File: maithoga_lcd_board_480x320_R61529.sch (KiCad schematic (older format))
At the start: 0 parts

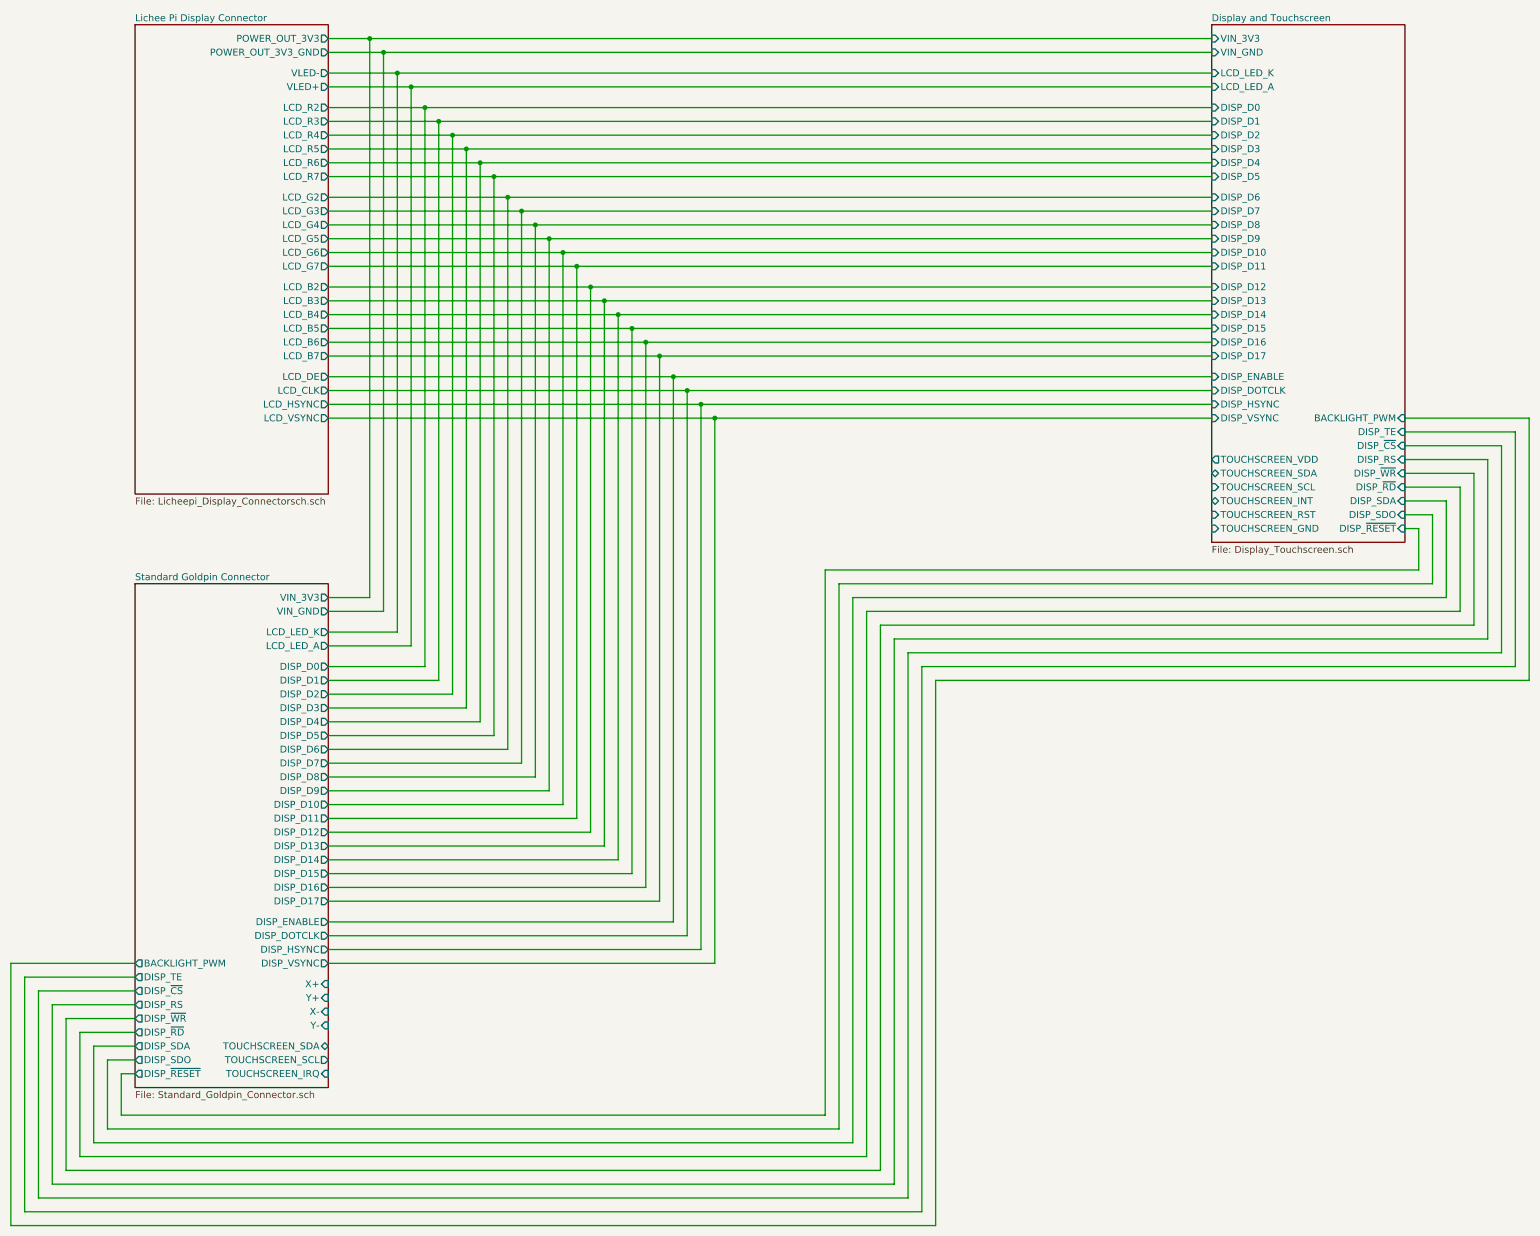
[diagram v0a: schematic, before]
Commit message: Generated gerbers
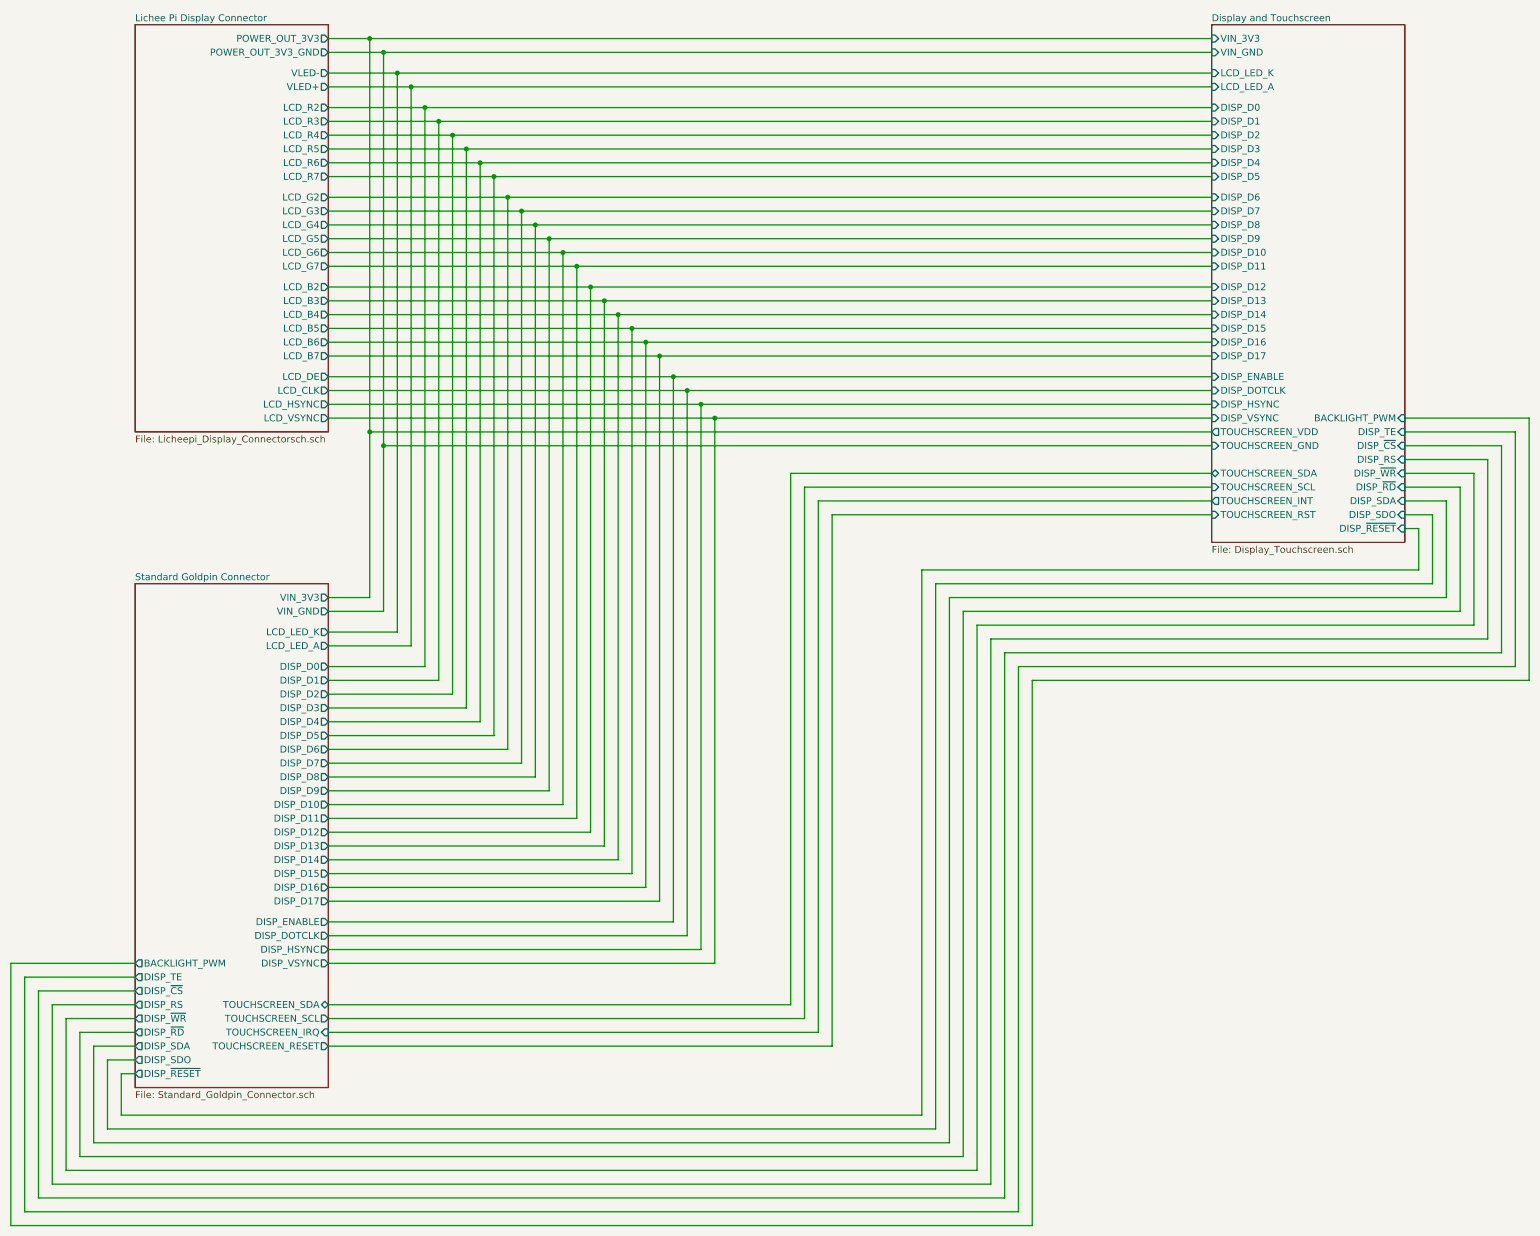
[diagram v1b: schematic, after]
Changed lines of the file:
@@
 F35 "LCD_LED_K" I L 11750 1800 50
 F36 "LCD_LED_A" I L 11750 1900 50
-F37 "TOUCHSCREEN_VDD" O L 11750 4600 50
+F37 "TOUCHSCREEN_VDD" O L 11750 4400 50
 F38 "TOUCHSCREEN_SDA" B L 11750 4700 50
 F39 "TOUCHSCREEN_SCL" I L 11750 4800 50
-F40 "TOUCHSCREEN_INT" B L 11750 4900 50
-F41 "TOUCHSCREEN_RST" I L 11750 5000 50
-F42 "TOUCHSCREEN_GND" I L 11750 5100 50
+F40 "TOUCHSCREEN_RST" I L 11750 5000 50
+F41 "TOUCHSCREEN_GND" I L 11750 4500 50
+F42 "TOUCHSCREEN_INT" O L 11750 4900 50
 $EndSheet
 $Sheet
@@
 F0 "Standard Goldpin Connector" 50
 F1 "Standard_Goldpin_Connector.sch" 50
-F2 "TOUCHSCREEN_IRQ" I R 5350 9050 50
-F3 "TOUCHSCREEN_SDA" B R 5350 8850 50
-F4 "TOUCHSCREEN_SCL" O R 5350 8950 50
-F5 "VIN_3V3" O R 5350 5600 50
-F6 "VIN_GND" O R 5350 5700 50
-F7 "BACKLIGHT_PWM" O L 3950 8250 50
-F8 "DISP_TE" O L 3950 8350 50
-F9 "DISP_~CS~" O L 3950 8450 50
-F10 "DISP_RS" O L 3950 8550 50
-F11 "DISP_~WR~" O L 3950 8650 50
-F12 "DISP_~RD~" O L 3950 8750 50
-F13 "DISP_SDA" O L 3950 8850 50
-F14 "DISP_SDO" O L 3950 8950 50
-F15 "DISP_D0" O R 5350 6100 50
-F16 "DISP_D1" O R 5350 6200 50
-F17 "DISP_D2" O R 5350 6300 50
-F18 "DISP_D3" O R 5350 6400 50
-F19 "DISP_D4" O R 5350 6500 50
-F20 "DISP_D5" O R 5350 6600 50
-F21 "DISP_D6" O R 5350 6700 50
-F22 "DISP_D7" O R 5350 6800 50
-F23 "DISP_D8" O R 5350 6900 50
-F24 "DISP_D9" O R 5350 7000 50
-F25 "DISP_D10" O R 5350 7100 50
-F26 "DISP_D11" O R 5350 7200 50
-F27 "DISP_D12" O R 5350 7300 50
-F28 "DISP_D13" O R 5350 7400 50
-F29 "DISP_D14" O R 5350 7500 50
-F30 "DISP_D15" O R 5350 7600 50
-F31 "DISP_D16" O R 5350 7700 50
-F32 "DISP_D17" O R 5350 7800 50
-F33 "DISP_ENABLE" O R 5350 7950 50
-F34 "DISP_DOTCLK" O R 5350 8050 50
-F35 "DISP_HSYNC" O R 5350 8150 50
-F36 "DISP_VSYNC" O R 5350 8250 50
-F37 "DISP_~RESET~" O L 3950 9050 50
-F38 "LCD_LED_K" O R 5350 5850 50
-F39 "LCD_LED_A" O R 5350 5950 50
-F40 "X-" I R 5350 8600 50
-F41 "X+" I R 5350 8400 50
-F42 "Y-" I R 5350 8700 50
-F43 "Y+" I R 5350 8500 50
+F2 "VIN_3V3" O R 5350 5600 50
+F3 "VIN_GND" O R 5350 5700 50
+F4 "BACKLIGHT_PWM" O L 3950 8250 50
+F5 "DISP_TE" O L 3950 8350 50
+F6 "DISP_~CS~" O L 3950 8450 50
+F7 "DISP_RS" O L 3950 8550 50
+F8 "DISP_~WR~" O L 3950 8650 50
+F9 "DISP_~RD~" O L 3950 8750 50
+F10 "DISP_SDA" O L 3950 8850 50
+F11 "DISP_SDO" O L 3950 8950 50
+F12 "DISP_D0" O R 5350 6100 50
+F13 "DISP_D1" O R 5350 6200 50
+F14 "DISP_D2" O R 5350 6300 50
+F15 "DISP_D3" O R 5350 6400 50
+F16 "DISP_D4" O R 5350 6500 50
+F17 "DISP_D5" O R 5350 6600 50
+F18 "DISP_D6" O R 5350 6700 50
+F19 "DISP_D7" O R 5350 6800 50
+F20 "DISP_D8" O R 5350 6900 50
+F21 "DISP_D9" O R 5350 7000 50
+F22 "DISP_D10" O R 5350 7100 50
+F23 "DISP_D11" O R 5350 7200 50
+F24 "DISP_D12" O R 5350 7300 50
+F25 "DISP_D13" O R 5350 7400 50
+F26 "DISP_D14" O R 5350 7500 50
+F27 "DISP_D15" O R 5350 7600 50
+F28 "DISP_D16" O R 5350 7700 50
+F29 "DISP_D17" O R 5350 7800 50
+F30 "DISP_ENABLE" O R 5350 7950 50
+F31 "DISP_DOTCLK" O R 5350 8050 50
+F32 "DISP_HSYNC" O R 5350 8150 50
+F33 "DISP_VSYNC" O R 5350 8250 50
+F34 "DISP_~RESET~" O L 3950 9050 50
+F35 "LCD_LED_K" O R 5350 5850 50
+F36 "LCD_LED_A" O R 5350 5950 50
+F37 "TOUCHSCREEN_IRQ" I R 5350 8750 50
+F38 "TOUCHSCREEN_SDA" B R 5350 8550 50
+F39 "TOUCHSCREEN_SCL" O R 5350 8650 50
+F40 "TOUCHSCREEN_RESET" O R 5350 8850 50
 $EndSheet
 $Sheet
-S 3950 1450 1400 3400
+S 3950 1450 1400 2950
 U 5F06906E
 F0 "Lichee Pi Display Connector" 50
@@
 Wire Wire Line
 	5350 5600 5650 5600
-Wire Wire Line
-	5650 5600 5650 1550
 Connection ~ 5650 1550
 Wire Wire Line
 	5650 1550 11750 1550
 Wire Wire Line
-	5750 1650 5750 5700
+	5750 1650 5750 4500
 Wire Wire Line
 	5750 5700 5350 5700
@@
 	13250 5100 13250 5400
 Wire Wire Line
-	8950 5400 8950 9350
-Wire Wire Line
-	8950 9350 3850 9350
+	9650 5400 9650 9350
+Wire Wire Line
+	9650 9350 3850 9350
 Wire Wire Line
 	3850 9350 3850 9050
@@
 	3850 9050 3950 9050
 Wire Wire Line
-	8950 5400 13250 5400
+	9650 5400 13250 5400
 Wire Wire Line
 	13150 5000 13350 5000
@@
 	13350 5000 13350 5500
 Wire Wire Line
-	13350 5500 9050 5500
-Wire Wire Line
-	9050 5500 9050 9450
-Wire Wire Line
-	9050 9450 3750 9450
+	13350 5500 9750 5500
+Wire Wire Line
+	9750 5500 9750 9450
+Wire Wire Line
+	9750 9450 3750 9450
 Wire Wire Line
 	3750 9450 3750 8950
@@
 	13450 4900 13450 5600
 Wire Wire Line
-	13450 5600 9150 5600
-Wire Wire Line
-	9150 5600 9150 9550
-Wire Wire Line
-	9150 9550 3650 9550
+	13450 5600 9850 5600
+Wire Wire Line
+	9850 5600 9850 9550
+Wire Wire Line
+	9850 9550 3650 9550
 Wire Wire Line
 	3650 9550 3650 8850
@@
 	13550 4800 13550 5700
 Wire Wire Line
-	13550 5700 9250 5700
-Wire Wire Line
-	9250 5700 9250 9650
-Wire Wire Line
-	9250 9650 3550 9650
+	13550 5700 9950 5700
+Wire Wire Line
+	9950 5700 9950 9650
+Wire Wire Line
+	9950 9650 3550 9650
 Wire Wire Line
 	3550 9650 3550 8750
@@
 	13650 4700 13650 5800
 Wire Wire Line
-	13650 5800 9350 5800
-Wire Wire Line
-	9350 5800 9350 9750
-Wire Wire Line
-	9350 9750 3450 9750
+	13650 5800 10050 5800
+Wire Wire Line
+	10050 5800 10050 9750
+Wire Wire Line
+	10050 9750 3450 9750
 Wire Wire Line
 	3450 9750 3450 8650
@@
 	13750 4600 13750 5900
 Wire Wire Line
-	13750 5900 9450 5900
-Wire Wire Line
-	9450 5900 9450 9850
-Wire Wire Line
-	9450 9850 3350 9850
+	13750 5900 10150 5900
+Wire Wire Line
+	10150 5900 10150 9850
+Wire Wire Line
+	10150 9850 3350 9850
 Wire Wire Line
 	3350 9850 3350 8550
@@
 	13850 4500 13850 6000
 Wire Wire Line
-	13850 6000 9550 6000
-Wire Wire Line
-	9550 6000 9550 9950
-Wire Wire Line
-	9550 9950 3250 9950
+	13850 6000 10250 6000
+Wire Wire Line
+	10250 6000 10250 9950
+Wire Wire Line
+	10250 9950 3250 9950
 Wire Wire Line
 	3250 9950 3250 8450
@@
 	13950 4400 13950 6100
 Wire Wire Line
-	13950 6100 9650 6100
-Wire Wire Line
-	9650 6100 9650 10050
-Wire Wire Line
-	9650 10050 3150 10050
+	13950 6100 10350 6100
+Wire Wire Line
+	10350 6100 10350 10050
+Wire Wire Line
+	10350 10050 3150 10050
 Wire Wire Line
 	3150 10050 3150 8350
@@
 	14050 4300 14050 6200
 Wire Wire Line
-	14050 6200 9750 6200
-Wire Wire Line
-	9750 6200 9750 10150
-Wire Wire Line
-	9750 10150 3050 10150
+	14050 6200 10450 6200
+Wire Wire Line
+	10450 6200 10450 10150
+Wire Wire Line
+	10450 10150 3050 10150
 Wire Wire Line
 	3050 10150 3050 8250
 Wire Wire Line
 	3050 8250 3950 8250
+Wire Wire Line
+	11750 4400 5650 4400
+Connection ~ 5650 4400
+Wire Wire Line
+	5650 4400 5650 1550
+Wire Wire Line
+	11750 4500 5750 4500
+Connection ~ 5750 4500
+Wire Wire Line
+	5350 8550 8700 8550
+Wire Wire Line
+	8700 8550 8700 4700
+Wire Wire Line
+	8700 4700 11750 4700
+Wire Wire Line
+	11750 4800 8800 4800
+Wire Wire Line
+	8800 4800 8800 8650
+Wire Wire Line
+	8800 8650 5350 8650
+Wire Wire Line
+	5350 8750 8900 8750
+Wire Wire Line
+	8900 8750 8900 4900
+Wire Wire Line
+	8900 4900 11750 4900
+Wire Wire Line
+	11750 5000 9000 5000
+Wire Wire Line
+	9000 5000 9000 8850
+Wire Wire Line
+	9000 8850 5350 8850
+Wire Wire Line
+	5650 4400 5650 5600
+Wire Wire Line
+	5750 4500 5750 5700
 $EndSCHEMATC
